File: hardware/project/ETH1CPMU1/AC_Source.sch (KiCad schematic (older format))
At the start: 97 parts, among them K801 TQ2SA-5V, U801 AD5453YRMZ, U802 LT1468, U803 LT1468, U804 AD9835, U805 ECS-3225SMV-500-GP-TR, U806 74AHCT1G08, U807 REF192, U808 TL071, U809 DG419LEUA, U810 TL072, U811 ADS7818, U812 AD5689BRUZ, U813 TL071, U814 TL072

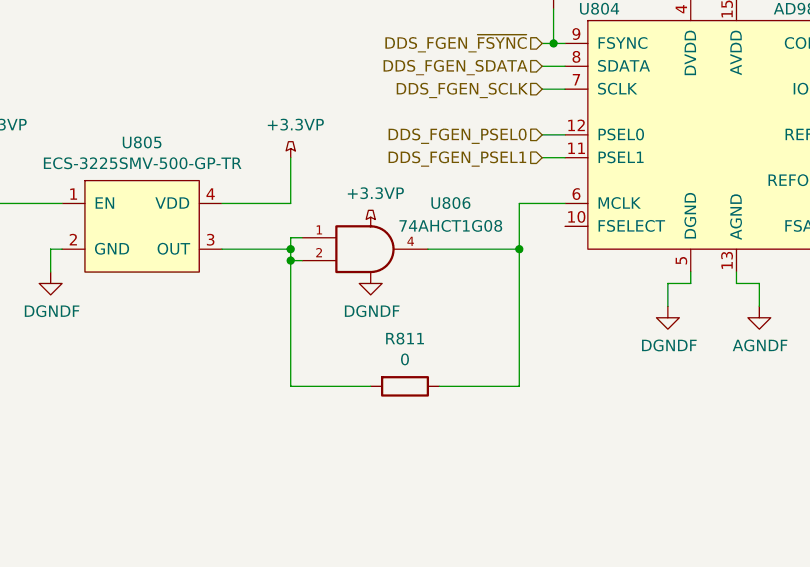
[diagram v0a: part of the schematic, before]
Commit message: Schematic and PCB design.
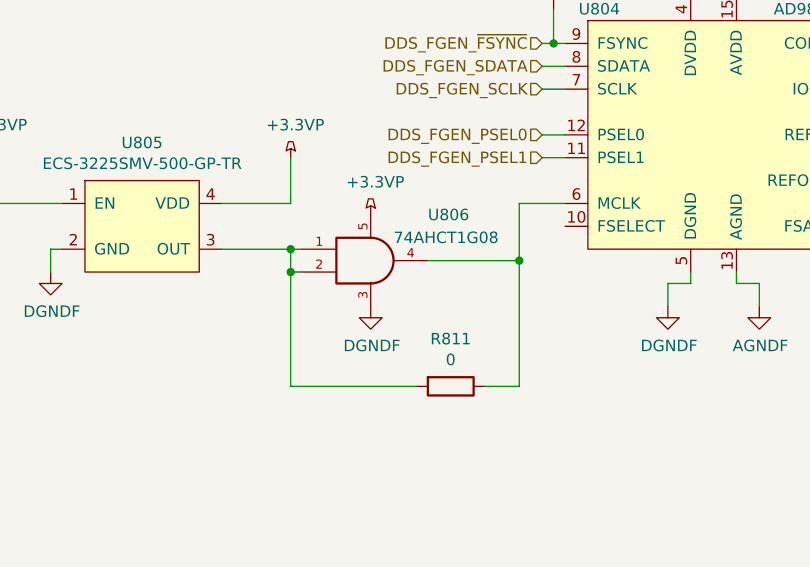
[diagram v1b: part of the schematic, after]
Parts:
- removed U806: 74AHCT1G08, Package_TO_SOT_SMD:SOT-23-5_HandSoldering, symbol 74xGxx:74AHCT1G08
- added U806: 74AHCT1G08, Package_TO_SOT_SMD:SOT-353_SC-70-5_Handsoldering, symbol ETH1CPMU1:74AHCT1G08
- U805: footprint (none) -> ETH1CPMU1:ECS
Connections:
- net +3.3VP: now also U806.5
- net DGNDF: now also U806.3
- net at R811.1, U804.6 (MCLK): now also U806.4
- net at R811.2, U805.3 (OUT): now also U806.1, U806.2
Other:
- moved on the sheet: R811
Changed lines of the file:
@@
 	5350 2200 4550 2200
 Connection ~ 5350 2200
-$Comp
-L 74xGxx:74AHCT1G08 U806
-U 1 1 5DD68372
-P 2400 2900
-F 0 "U806" H 2750 3100 50  0000 C CNN
-F 1 "74AHCT1G08" H 2750 3000 50  0000 C CNN
-F 2 "Package_TO_SOT_SMD:SOT-23-5_HandSoldering" H 2400 2900 50  0001 C CNN
-F 3 "http://www.ti.com/lit/sg/scyt129e/scyt129e.pdf" H 2400 2900 50  0001 C CNN
-	1    2400 2900
-	1    0    0    -1
-$EndComp
-Wire Wire Line
-	2650 2900 3050 2900
-$Comp
-L ETH1CPMU1:DGNDF #PWR0824
-U 1 1 5DD7B574
-P 2400 3000
-F 0 "#PWR0824" H 2400 2750 50  0001 C CNN
-F 1 "DGNDF" H 2405 2827 50  0000 C CNN
-F 2 "" H 2400 3000 50  0001 C CNN
-F 3 "" H 2400 3000 50  0001 C CNN
-	1    2400 3000
-	1    0    0    -1
-$EndComp
-Wire Wire Line
-	2100 2950 2050 2950
-Wire Wire Line
-	2050 2850 2100 2850
-Wire Wire Line
-	2050 2850 2050 2900
-Wire Wire Line
-	3050 2900 3050 2700
+Wire Wire Line
+	2650 2950 3050 2950
+Wire Wire Line
+	2100 3000 2050 3000
+Wire Wire Line
+	2050 2900 2100 2900
+Wire Wire Line
+	3050 2950 3050 2700
 Wire Wire Line
 	3050 2700 3250 2700
@@
 F 0 "U805" H 1400 3165 50  0000 C CNN
 F 1 "ECS-3225SMV-500-GP-TR" H 1400 3074 50  0000 C CNN
-F 2 "" H 1800 3350 50  0001 C CNN
+F 2 "ETH1CPMU1:ECS" H 1800 3350 50  0001 C CNN
 F 3 "" H 1800 3350 50  0001 C CNN
 	1    1400 2800
@@
 Connection ~ 2050 2900
 Wire Wire Line
-	2050 2900 2050 2950
+	2050 2900 2050 3000
 $Comp
 L ETH1CPMU1:DGNDF #PWR0823
@@
 	1    0    0    -1
 $EndComp
-$Comp
-L power:+3.3VP #PWR0822
-U 1 1 5F50A5E2
-P 2400 2800
-F 0 "#PWR0822" H 2550 2750 50  0001 C CNN
-F 1 "+3.3VP" H 2420 2943 50  0000 C CNN
-F 2 "" H 2400 2800 50  0001 C CNN
-F 3 "" H 2400 2800 50  0001 C CNN
-	1    2400 2800
-	1    0    0    -1
-$EndComp
 Text HLabel 15050 2400 2    50   Output ~ 0
 AC_FOURCE
@@
 L Device:R R811
 U 1 1 5DD89B99
-P 2550 3500
-F 0 "R811" V 2343 3500 50  0000 C CNN
-F 1 "0" V 2434 3500 50  0000 C CNN
-F 2 "Resistor_SMD:R_0603_1608Metric_Pad1.05x0.95mm_HandSolder" V 2480 3500 50  0001 C CNN
-F 3 "~" H 2550 3500 50  0001 C CNN
-	1    2550 3500
-	0    1    1    0
-$EndComp
-Wire Wire Line
-	2400 3500 2050 3500
-Wire Wire Line
-	2050 3500 2050 2950
-Connection ~ 2050 2950
-Wire Wire Line
-	2700 3500 3050 3500
-Wire Wire Line
-	3050 3500 3050 2900
-Connection ~ 3050 2900
+P 2750 3500
+F 0 "R811" V 2543 3500 50  0000 C CNN
+F 1 "0" V 2634 3500 50  0000 C CNN
+F 2 "Resistor_SMD:R_0603_1608Metric_Pad1.05x0.95mm_HandSolder" V 2680 3500 50  0001 C CNN
+F 3 "~" H 2750 3500 50  0001 C CNN
+	1    2750 3500
+	0    1    1    0
+$EndComp
+Wire Wire Line
+	2600 3500 2050 3500
+Wire Wire Line
+	2050 3500 2050 3000
+Connection ~ 2050 3000
+Wire Wire Line
+	2900 3500 3050 3500
+Wire Wire Line
+	3050 3500 3050 2950
+Connection ~ 3050 2950
 $Comp
 L Device:R R806
@@
 	13250 2300 12800 2300
 Connection ~ 12800 2300
-Wire Wire Line
-	13850 2400 15050 2400
 $Comp
 L Amplifier_Operational:TL072 U810
@@
 Text Label 4650 8000 0    50   ~ 0
 +2V5REF
+Wire Wire Line
+	13850 2400 15050 2400
+$Comp
+L ETH1CPMU1:74AHCT1G08 U806
+U 1 1 5E75FDEB
+P 2400 2950
+F 0 "U806" H 2650 3150 50  0000 L CNN
+F 1 "74AHCT1G08" H 2500 3050 50  0000 L CNN
+F 2 "Package_TO_SOT_SMD:SOT-353_SC-70-5_Handsoldering" H 2400 2950 50  0001 C CNN
+F 3 "http://www.ti.com/lit/sg/scyt129e/scyt129e.pdf" H 2400 2950 50  0001 C CNN
+	1    2400 2950
+	1    0    0    -1
+$EndComp
+$Comp
+L power:+3.3VP #PWR0822
+U 1 1 5E761278
+P 2400 2750
+F 0 "#PWR0822" H 2550 2700 50  0001 C CNN
+F 1 "+3.3VP" H 2420 2893 50  0000 C CNN
+F 2 "" H 2400 2750 50  0001 C CNN
+F 3 "" H 2400 2750 50  0001 C CNN
+	1    2400 2750
+	1    0    0    -1
+$EndComp
+$Comp
+L ETH1CPMU1:DGNDF #PWR0824
+U 1 1 5E7D5BEA
+P 2400 3150
+F 0 "#PWR0824" H 2400 2900 50  0001 C CNN
+F 1 "DGNDF" H 2405 2977 50  0000 C CNN
+F 2 "" H 2400 3150 50  0001 C CNN
+F 3 "" H 2400 3150 50  0001 C CNN
+	1    2400 3150
+	1    0    0    -1
+$EndComp
 $EndSCHEMATC
